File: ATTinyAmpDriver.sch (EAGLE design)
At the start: 34 parts, among them Q1 SI2301CDS, Q2 BC846, U1 SPX5205M5-L-3-3, U2 ATTINY5-TSHR, U3 MCP6L2-X_SN, X2 INPUT

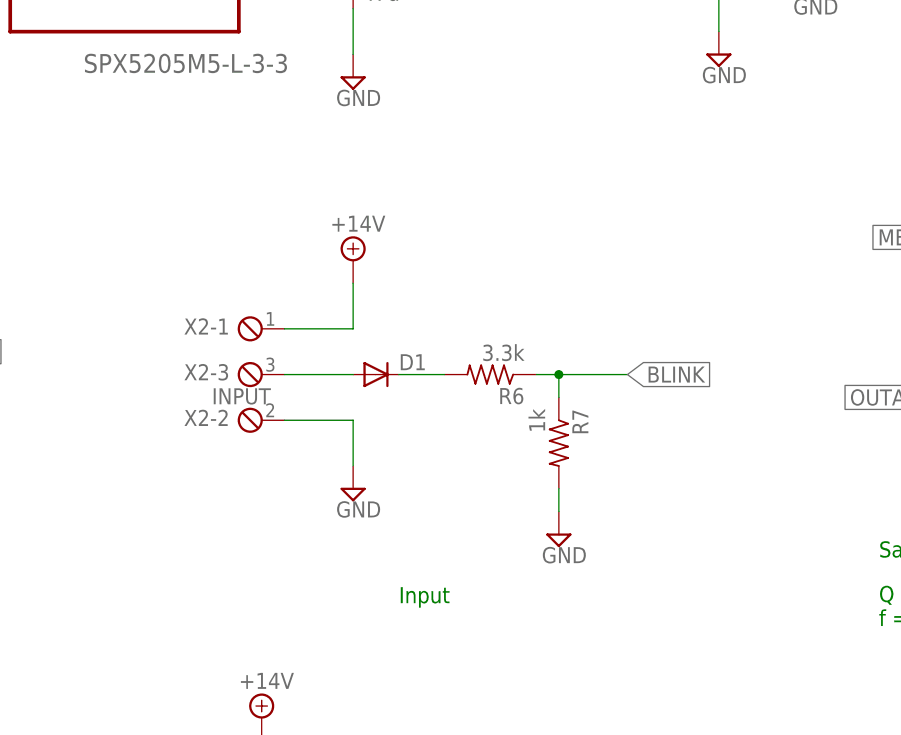
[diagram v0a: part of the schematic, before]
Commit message: Board Complete
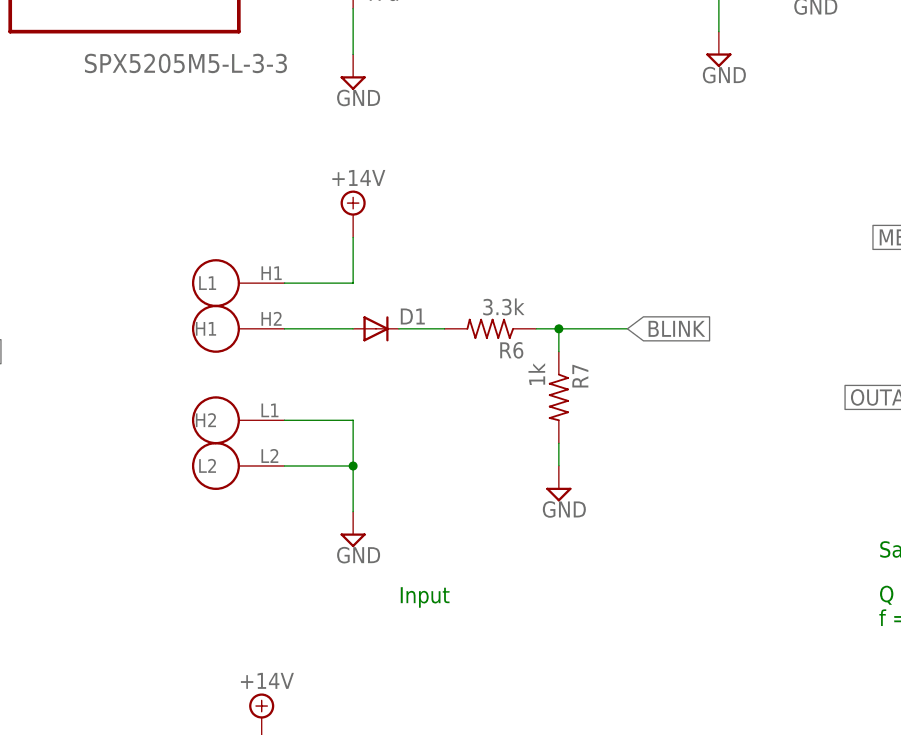
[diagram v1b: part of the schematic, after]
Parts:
- removed X2: INPUT, con-phoenix-254:MPT3
- added U$1: CON_TAILLIGHT, Combined:CON_TAILLIGHT
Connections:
- net +14V: now also U$1.L1; no longer X2-1.1
- net GND: now also U$1.H2, U$1.L2; no longer X2-2.1
- net N$1: now also U$1.H1; no longer X2-3.1
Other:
- moved on the sheet: D1, R6, R7
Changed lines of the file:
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@@
 <attribute name="DIGIKEY_COST" value=".60"/>
 </part>
-<part name="X2" library="con-phoenix-254" deviceset="MPT3" device="" value="INPUT"/>
 <part name="SUPPLY1" library="supply2" deviceset="+14V" device=""/>
 <part name="SUPPLY2" library="supply2" deviceset="GND" device=""/>
@@
 <part name="LED4" library="Combined" deviceset="LUXEON_REBEL" device="CREE_XP-E"/>
 <part name="SUPPLY20" library="supply2" deviceset="GND" device=""/>
+<part name="U$1" library="Combined" deviceset="CON_TAILLIGHT" device=""/>
 </parts>
 <sheets>
@@
 <attribute name="DIGIKEY_COST" x="66.04" y="180.34" size="1.778" layer="96" display="off"/>
 </instance>
-<instance part="X2" gate="-1" x="81.28" y="132.08" rot="MR0"/>
-<instance part="X2" gate="-2" x="81.28" y="121.92" rot="MR0"/>
-<instance part="X2" gate="-3" x="81.28" y="127" rot="MR0"/>
-<instance part="SUPPLY1" gate="G$1" x="91.44" y="139.7"/>
-<instance part="SUPPLY2" gate="GND" x="91.44" y="114.3"/>
+<instance part="SUPPLY1" gate="G$1" x="91.44" y="144.78"/>
+<instance part="SUPPLY2" gate="GND" x="91.44" y="109.22"/>
 <instance part="SUPPLY3" gate="G$1" x="96.52" y="195.58"/>
 <instance part="C3" gate="G$1" x="91.44" y="172.72">
@@
 </instance>
 <instance part="SUPPLY9" gate="G$1" x="38.1" y="195.58"/>
-<instance part="R6" gate="G$1" x="106.68" y="127" rot="R180">
-<attribute name="DIGIKEY" x="106.68" y="127" size="1.778" layer="96" rot="R180" display="off"/>
-<attribute name="DIGIKEY_COST" x="106.68" y="127" size="1.778" layer="96" rot="R180" display="off"/>
-</instance>
-<instance part="R7" gate="G$1" x="114.3" y="119.38" rot="R270">
-<attribute name="DIGIKEY" x="114.3" y="119.38" size="1.778" layer="96" rot="R270" display="off"/>
-<attribute name="DIGIKEY_COST" x="114.3" y="119.38" size="1.778" layer="96" rot="R270" display="off"/>
-</instance>
-<instance part="SUPPLY10" gate="GND" x="114.3" y="109.22"/>
+<instance part="R6" gate="G$1" x="106.68" y="132.08" rot="R180">
+<attribute name="DIGIKEY" x="106.68" y="132.08" size="1.778" layer="96" rot="R180" display="off"/>
+<attribute name="DIGIKEY_COST" x="106.68" y="132.08" size="1.778" layer="96" rot="R180" display="off"/>
+</instance>
+<instance part="R7" gate="G$1" x="114.3" y="124.46" rot="R270">
+<attribute name="DIGIKEY" x="114.3" y="124.46" size="1.778" layer="96" rot="R270" display="off"/>
+<attribute name="DIGIKEY_COST" x="114.3" y="124.46" size="1.778" layer="96" rot="R270" display="off"/>
+</instance>
+<instance part="SUPPLY10" gate="GND" x="114.3" y="114.3"/>
 <instance part="R2" gate="G$1" x="58.42" y="73.66" rot="MR270">
 <attribute name="DIGIKEY" x="58.42" y="73.66" size="1.778" layer="96" rot="MR270" display="off"/>
@@
 </instance>
 <instance part="SUPPLY22" gate="GND" x="243.84" y="35.56"/>
-<instance part="D1" gate="G$1" x="93.98" y="127" smashed="yes">
-<attribute name="DIGIKEY" x="93.98" y="127" size="1.778" layer="96" display="off"/>
-<attribute name="DIGIKEY_COST" x="93.98" y="127" size="1.778" layer="96" display="off"/>
-<attribute name="NAME" x="96.52" y="127.4826" size="1.778" layer="95"/>
+<instance part="D1" gate="G$1" x="93.98" y="132.08" smashed="yes">
+<attribute name="DIGIKEY" x="93.98" y="132.08" size="1.778" layer="96" display="off"/>
+<attribute name="DIGIKEY_COST" x="93.98" y="132.08" size="1.778" layer="96" display="off"/>
+<attribute name="NAME" x="96.52" y="132.5626" size="1.778" layer="95"/>
 </instance>
 <instance part="R8" gate="G$1" x="228.6" y="124.46" rot="MR270">
@@
 <instance part="LED4" gate="TH" x="149.86" y="30.48" rot="R180"/>
 <instance part="SUPPLY20" gate="GND" x="134.62" y="15.24"/>
+<instance part="U$1" gate="G$1" x="83.82" y="127"/>
 </instances>
 <busses>
@@
 <segment>
 <pinref part="SUPPLY2" gate="GND" pin="GND"/>
+<wire x1="91.44" y1="116.84" x2="91.44" y2="111.76" width="0.1524" layer="91"/>
+<wire x1="83.82" y1="116.84" x2="91.44" y2="116.84" width="0.1524" layer="91"/>
+<pinref part="U$1" gate="G$1" pin="L2"/>
+<pinref part="U$1" gate="G$1" pin="H2"/>
+<wire x1="83.82" y1="121.92" x2="91.44" y2="121.92" width="0.1524" layer="91"/>
 <wire x1="91.44" y1="121.92" x2="91.44" y2="116.84" width="0.1524" layer="91"/>
-<pinref part="X2" gate="-2" pin="1"/>
-<wire x1="83.82" y1="121.92" x2="91.44" y2="121.92" width="0.1524" layer="91"/>
+<junction x="91.44" y="116.84"/>
 </segment>
 <segment>
@@
 <pinref part="R7" gate="G$1" pin="2"/>
 <pinref part="SUPPLY10" gate="GND" pin="GND"/>
-<wire x1="114.3" y1="114.3" x2="114.3" y2="111.76" width="0.1524" layer="91"/>
+<wire x1="114.3" y1="119.38" x2="114.3" y2="116.84" width="0.1524" layer="91"/>
 </segment>
 <segment>
@@
 <net name="+14V" class="0">
 <segment>
-<pinref part="X2" gate="-1" pin="1"/>
 <pinref part="SUPPLY1" gate="G$1" pin="+14V"/>
-<wire x1="83.82" y1="132.08" x2="91.44" y2="132.08" width="0.1524" layer="91"/>
-<wire x1="91.44" y1="132.08" x2="91.44" y2="137.16" width="0.1524" layer="91"/>
+<wire x1="83.82" y1="137.16" x2="91.44" y2="137.16" width="0.1524" layer="91"/>
+<wire x1="91.44" y1="137.16" x2="91.44" y2="142.24" width="0.1524" layer="91"/>
+<pinref part="U$1" gate="G$1" pin="L1"/>
 </segment>
 <segment>
@@
 <segment>
 <pinref part="R6" gate="G$1" pin="1"/>
-<wire x1="111.76" y1="127" x2="114.3" y2="127" width="0.1524" layer="91"/>
+<wire x1="111.76" y1="132.08" x2="114.3" y2="132.08" width="0.1524" layer="91"/>
 <pinref part="R7" gate="G$1" pin="1"/>
-<wire x1="114.3" y1="127" x2="121.92" y2="127" width="0.1524" layer="91"/>
-<wire x1="114.3" y1="124.46" x2="114.3" y2="127" width="0.1524" layer="91"/>
-<junction x="114.3" y="127"/>
-<label x="121.92" y="127" size="1.778" layer="95" xref="yes"/>
+<wire x1="114.3" y1="132.08" x2="121.92" y2="132.08" width="0.1524" layer="91"/>
+<wire x1="114.3" y1="129.54" x2="114.3" y2="132.08" width="0.1524" layer="91"/>
+<junction x="114.3" y="132.08"/>
+<label x="121.92" y="132.08" size="1.778" layer="95" xref="yes"/>
 </segment>
 <segment>
@@
 <net name="N$1" class="0">
 <segment>
-<pinref part="X2" gate="-3" pin="1"/>
 <pinref part="D1" gate="G$1" pin="A"/>
-<wire x1="83.82" y1="127" x2="91.44" y2="127" width="0.1524" layer="91"/>
+<wire x1="83.82" y1="132.08" x2="91.44" y2="132.08" width="0.1524" layer="91"/>
+<pinref part="U$1" gate="G$1" pin="H1"/>
 </segment>
 </net>
@@
 <pinref part="D1" gate="G$1" pin="C"/>
 <pinref part="R6" gate="G$1" pin="2"/>
-<wire x1="96.52" y1="127" x2="101.6" y2="127" width="0.1524" layer="91"/>
-</segment>
-</net>
+<wire x1="96.52" y1="132.08" x2="101.6" y2="132.08" width="0.1524" layer="91"/>
+</segment>
+</net>
